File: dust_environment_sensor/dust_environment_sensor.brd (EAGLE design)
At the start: 60 x 34 mm, 4 parts, among them U1 LTP5901, U2 LIS3DH, U3 SI7005, U4 TSL2560

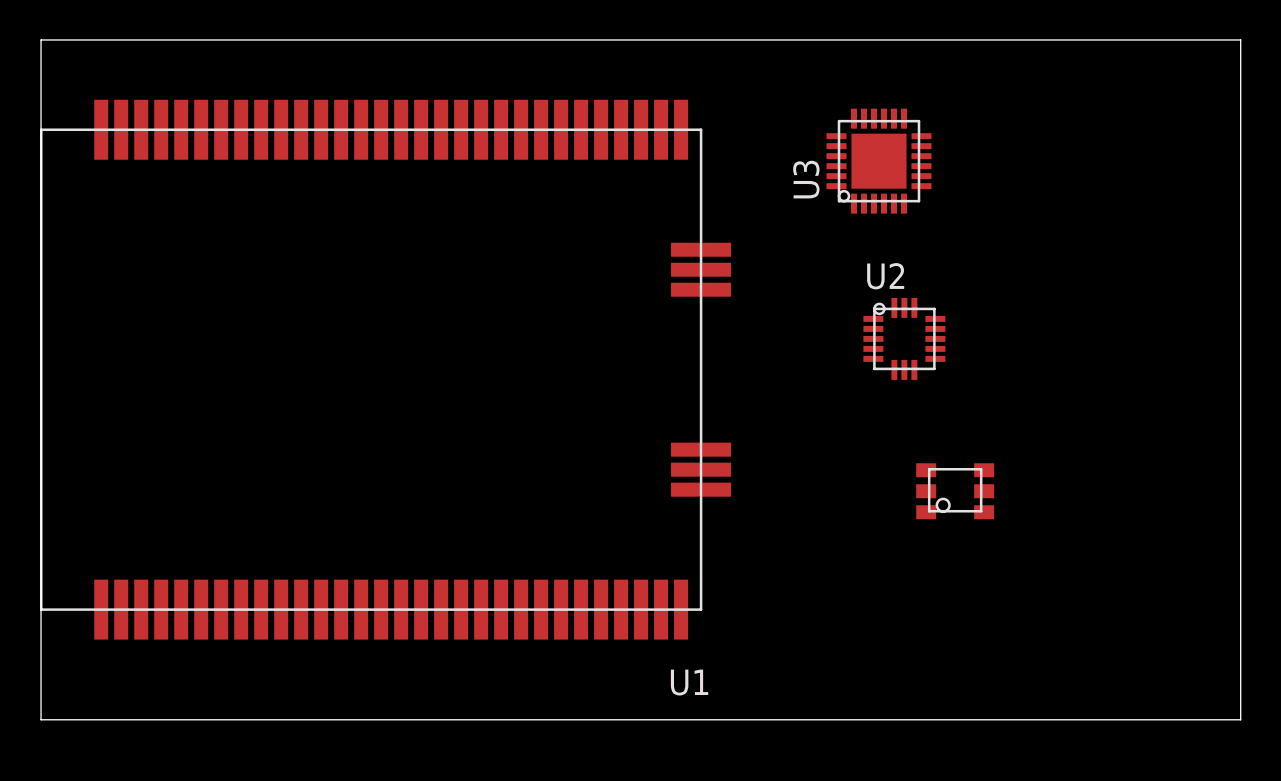
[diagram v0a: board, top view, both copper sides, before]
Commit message: Battery holder
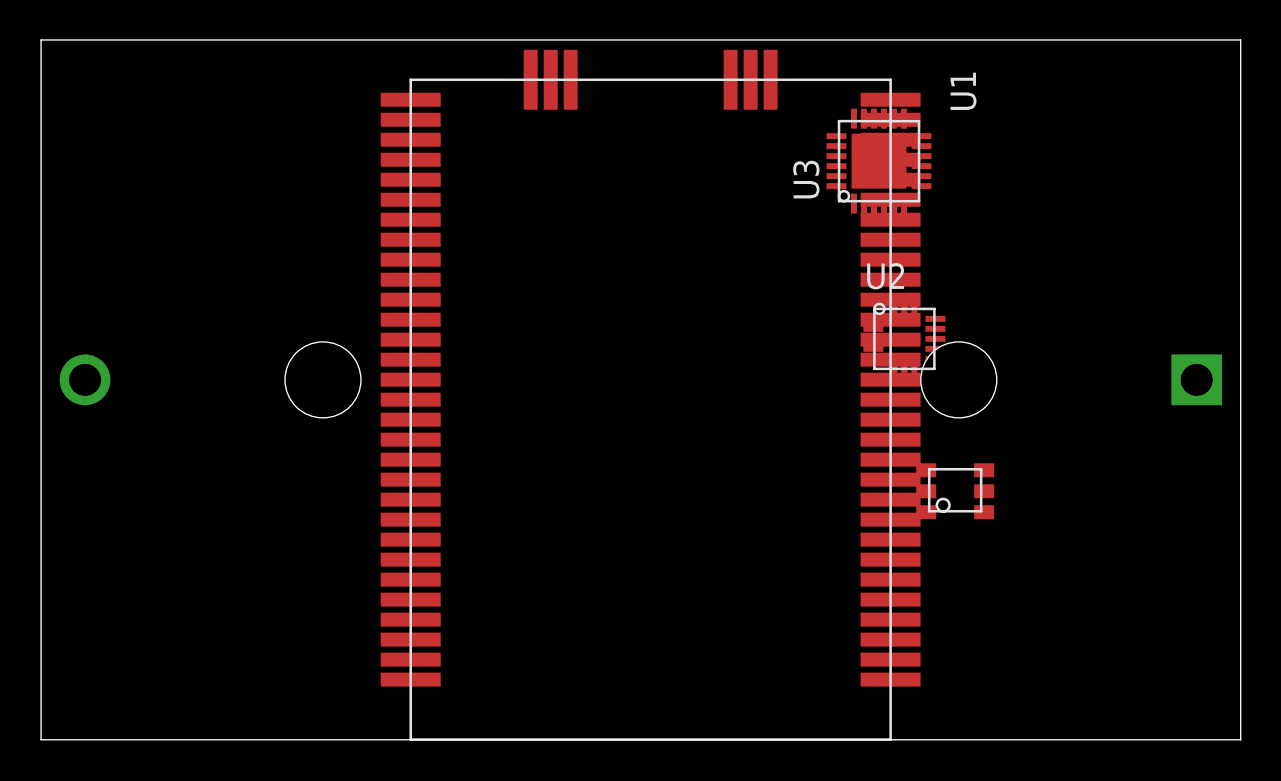
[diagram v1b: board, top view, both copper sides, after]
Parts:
- added J1: (no value), Cool_Electricity:BX0036
- moved U1 14.1 mm to (30.5, 15.5), turned to 180 degrees
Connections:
- net GND: now also J1.NEG
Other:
- board size 60 x 34 mm -> 60 x 35 mm
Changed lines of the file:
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@@
 <board>
 <plain>
-<wire x1="0" y1="0" x2="60" y2="0" width="0" layer="20"/>
-<wire x1="60" y1="0" x2="60" y2="34" width="0" layer="20"/>
+<wire x1="0" y1="-1" x2="60" y2="-1" width="0" layer="20"/>
+<wire x1="60" y1="-1" x2="60" y2="34" width="0" layer="20"/>
 <wire x1="60" y1="34" x2="0" y2="34" width="0" layer="20"/>
-<wire x1="0" y1="34" x2="0" y2="0" width="0" layer="20"/>
+<wire x1="0" y1="34" x2="0" y2="-1" width="0" layer="20"/>
 </plain>
 <attributes>
@@
 </autorouter>
 <elements>
-<element name="U1" library="Cool_Electricity" package="LTP5901_MODULE" value="LTP5901" x="16.51" y="17.51" rot="R90"/>
+<element name="U1" library="Cool_Electricity" package="LTP5901_MODULE" value="LTP5901" x="30.49" y="15.51" rot="R180"/>
 <element name="U2" library="Cool_Electricity" package="LGA16_ST" value="LIS3DH" x="43.18" y="19.05"/>
 <element name="U3" library="Cool_Electricity" package="QFN24_SILICON_LABS" value="SI7005" x="41.91" y="27.94" rot="R90"/>
 <element name="U4" library="Cool_Electricity" package="CL6_TAOS" value="TSL2560" x="45.72" y="11.43"/>
+<element name="J1" library="Cool_Electricity" package="BX0036" value="" x="30" y="17" rot="MR0"/>
 </elements>
 <signals>
@@
 <contactref element="U2" pad="12"/>
 <contactref element="U2" pad="10"/>
-<wire x1="22.01" y1="5.51" x2="32.01" y2="5.51" width="0" layer="19" extent="1-1"/>
-<wire x1="13.01" y1="5.51" x2="22.01" y2="5.51" width="0" layer="19" extent="1-1"/>
-<wire x1="3.01" y1="5.51" x2="13.01" y2="5.51" width="0" layer="19" extent="1-1"/>
-<wire x1="33.01" y1="21.51" x2="32.01" y2="5.51" width="0" layer="19" extent="1-1"/>
-<wire x1="32.01" y1="29.51" x2="33.01" y2="21.51" width="0" layer="19" extent="1-1"/>
-<wire x1="27.01" y1="29.51" x2="32.01" y2="29.51" width="0" layer="19" extent="1-1"/>
-<wire x1="13.01" y1="29.51" x2="27.01" y2="29.51" width="0" layer="19" extent="1-1"/>
-<wire x1="3.01" y1="29.51" x2="13.01" y2="29.51" width="0" layer="19" extent="1-1"/>
-<wire x1="44.035" y1="28.69" x2="3.01" y2="29.51" width="0" layer="19" extent="1-1"/>
+<contactref element="J1" pad="NEG"/>
 <wire x1="44.035" y1="27.19" x2="44.035" y2="28.69" width="0" layer="19" extent="1-1"/>
 <wire x1="41.91" y1="27.94" x2="44.035" y2="28.69" width="0" layer="19" extent="1-1"/>
+<wire x1="40.66" y1="25.815" x2="41.91" y2="27.94" width="0" layer="19" extent="1-1"/>
 <wire x1="39.785" y1="29.19" x2="41.91" y2="27.94" width="0" layer="19" extent="1-1"/>
-<wire x1="40.66" y1="25.815" x2="41.91" y2="27.94" width="0" layer="19" extent="1-1"/>
 <wire x1="44.73" y1="19.55" x2="40.66" y2="25.815" width="0" layer="19" extent="1-1"/>
 <wire x1="44.73" y1="18.55" x2="44.73" y2="19.55" width="0" layer="19" extent="1-1"/>
 <wire x1="41.63" y1="18.05" x2="44.73" y2="18.55" width="0" layer="19" extent="1-1"/>
+<wire x1="18.49" y1="31.01" x2="39.785" y2="29.19" width="0" layer="19" extent="1-1"/>
+<wire x1="18.49" y1="26.01" x2="18.49" y2="31.01" width="0" layer="19" extent="1-1"/>
+<wire x1="26.49" y1="32.01" x2="18.49" y2="31.01" width="0" layer="19" extent="1-1"/>
+<wire x1="18.49" y1="12.01" x2="18.49" y2="26.01" width="0" layer="19" extent="1-1"/>
+<wire x1="18.49" y1="2.01" x2="18.49" y2="12.01" width="0" layer="19" extent="1-1"/>
+<wire x1="42.49" y1="31.01" x2="41.63" y2="18.05" width="0" layer="19" extent="1-1"/>
+<wire x1="42.49" y1="21.01" x2="42.49" y2="31.01" width="0" layer="19" extent="1-1"/>
+<wire x1="42.49" y1="12.01" x2="42.49" y2="21.01" width="0" layer="19" extent="1-1"/>
+<wire x1="42.49" y1="2.01" x2="42.49" y2="12.01" width="0" layer="19" extent="1-1"/>
+<wire x1="2.2" y1="17" x2="42.49" y2="31.01" width="0" layer="19" extent="1-1"/>
 </signal>
 </signals>
